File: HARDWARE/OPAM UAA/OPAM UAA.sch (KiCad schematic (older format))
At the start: 20 parts, among them J1 BATT+, J2 CELDA, U1 LM317L_TO92, U2 LM324A, U3 LM35-LP, U4 LM35-LP

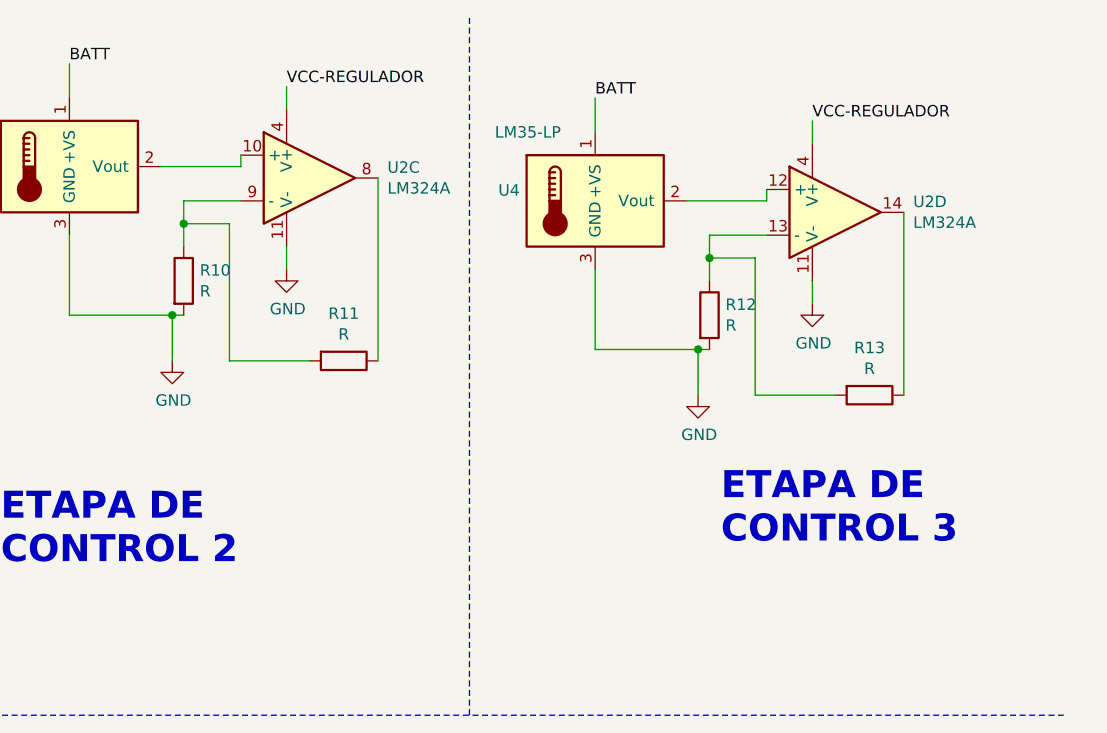
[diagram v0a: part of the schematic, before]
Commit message: PCB 2.0
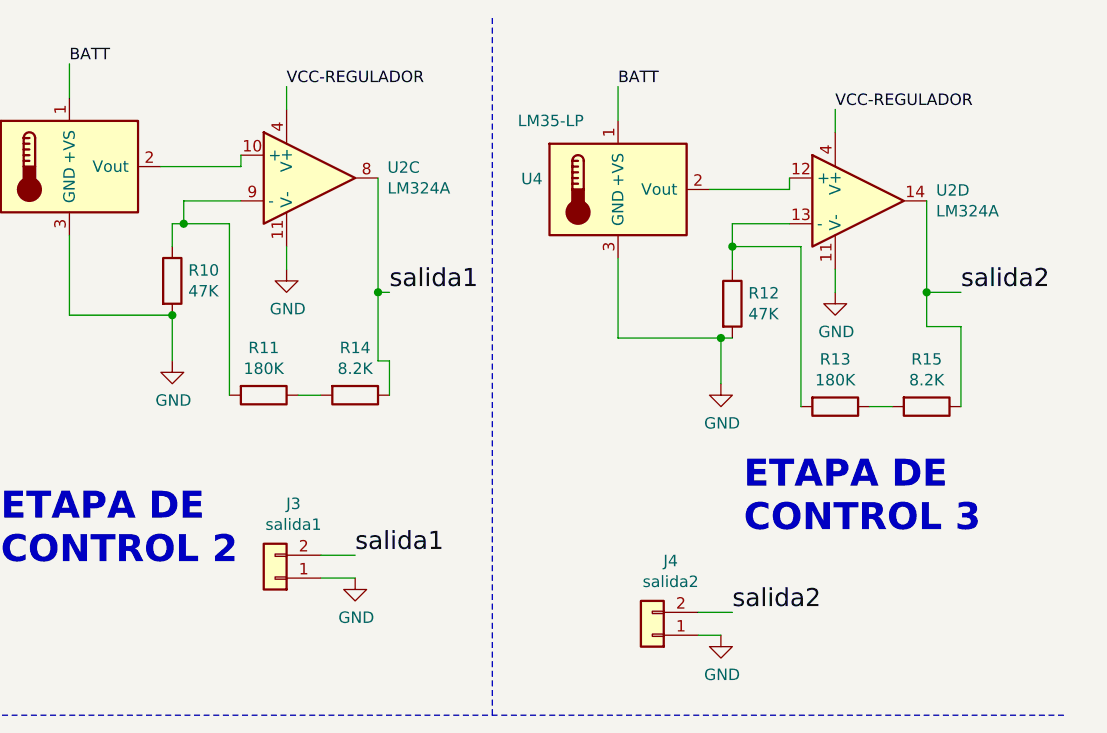
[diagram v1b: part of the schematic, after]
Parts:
- added J3: salida1, Pin_Headers:Pin_Header_Straight_1x02_Pitch2.54mm, symbol conn:Conn_01x02
- added J4: salida2, Pin_Headers:Pin_Header_Straight_1x02_Pitch2.54mm, symbol conn:Conn_01x02
- added R14, R15: 8.2K, Resistors_THT:R_Axial_DIN0411_L9.9mm_D3.6mm_P12.70mm_Horizontal, symbol device:R
- J1, J2: footprint (none) -> Pin_Headers:Pin_Header_Straight_1x02_Pitch2.54mm
- R1, R2, R3, R4, R5, R6, R7, R8, R9: footprint (none) -> Resistors_THT:R_Axial_DIN0411_L9.9mm_D3.6mm_P12.70mm_Horizontal
- R10, R12: value R -> 47K; footprint (none) -> Resistors_THT:R_Axial_DIN0411_L9.9mm_D3.6mm_P12.70mm_Horizontal
- R11, R13: value R -> 180K; footprint (none) -> Resistors_THT:R_Axial_DIN0411_L9.9mm_D3.6mm_P12.70mm_Horizontal
- RV1: footprint (none) -> Potentiometers:Potentiometer_WirePads_largePads
- U1: footprint TO_SOT_Packages_THT:TO-92_Inline_Narrow_Oval -> TO_SOT_Packages_THT:TO-92_Inline_Wide
- U2: footprint (none) -> Housings_DIP:DIP-14_W7.62mm_Socket_LongPads
- U3, U4: footprint (none) -> TO_SOT_Packages_THT:TO-92_Inline_Narrow_Oval
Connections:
- net GND: now also J3.1 (Pin_1), J4.1 (Pin_1)
- net at R11.1: now also R14.2; no longer U2.8
- net at R13.1: now also R15.2; no longer U2.14
- new net salida1: J3.2 (Pin_2), R14.1, U2.8
- new net salida2: J4.2 (Pin_2), R15.1, U2.14
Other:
- moved on the sheet: R10, R11, R12, R13, U2D, U4
